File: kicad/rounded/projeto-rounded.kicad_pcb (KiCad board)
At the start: 2 copper layers, 123.2 x 127 mm, 57 parts, among them Q1 BTA16-600B, Q2 BTA16-600B, U1 ESP-12E, U3v3 LM1117-3.3

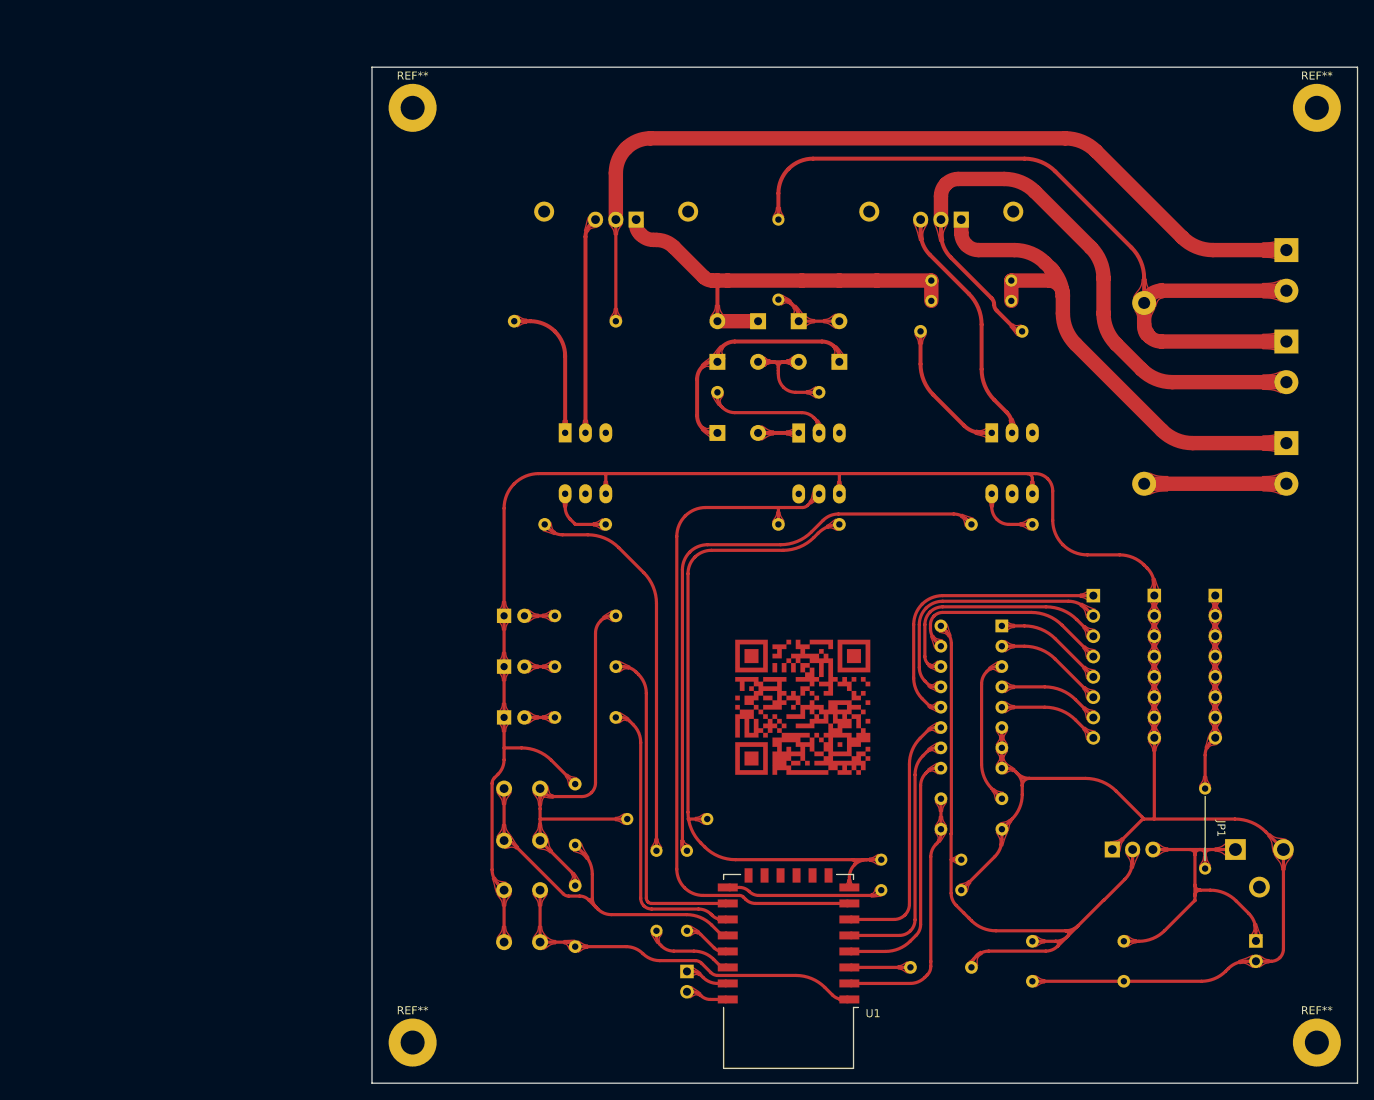
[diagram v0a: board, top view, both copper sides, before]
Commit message: Fix PCB
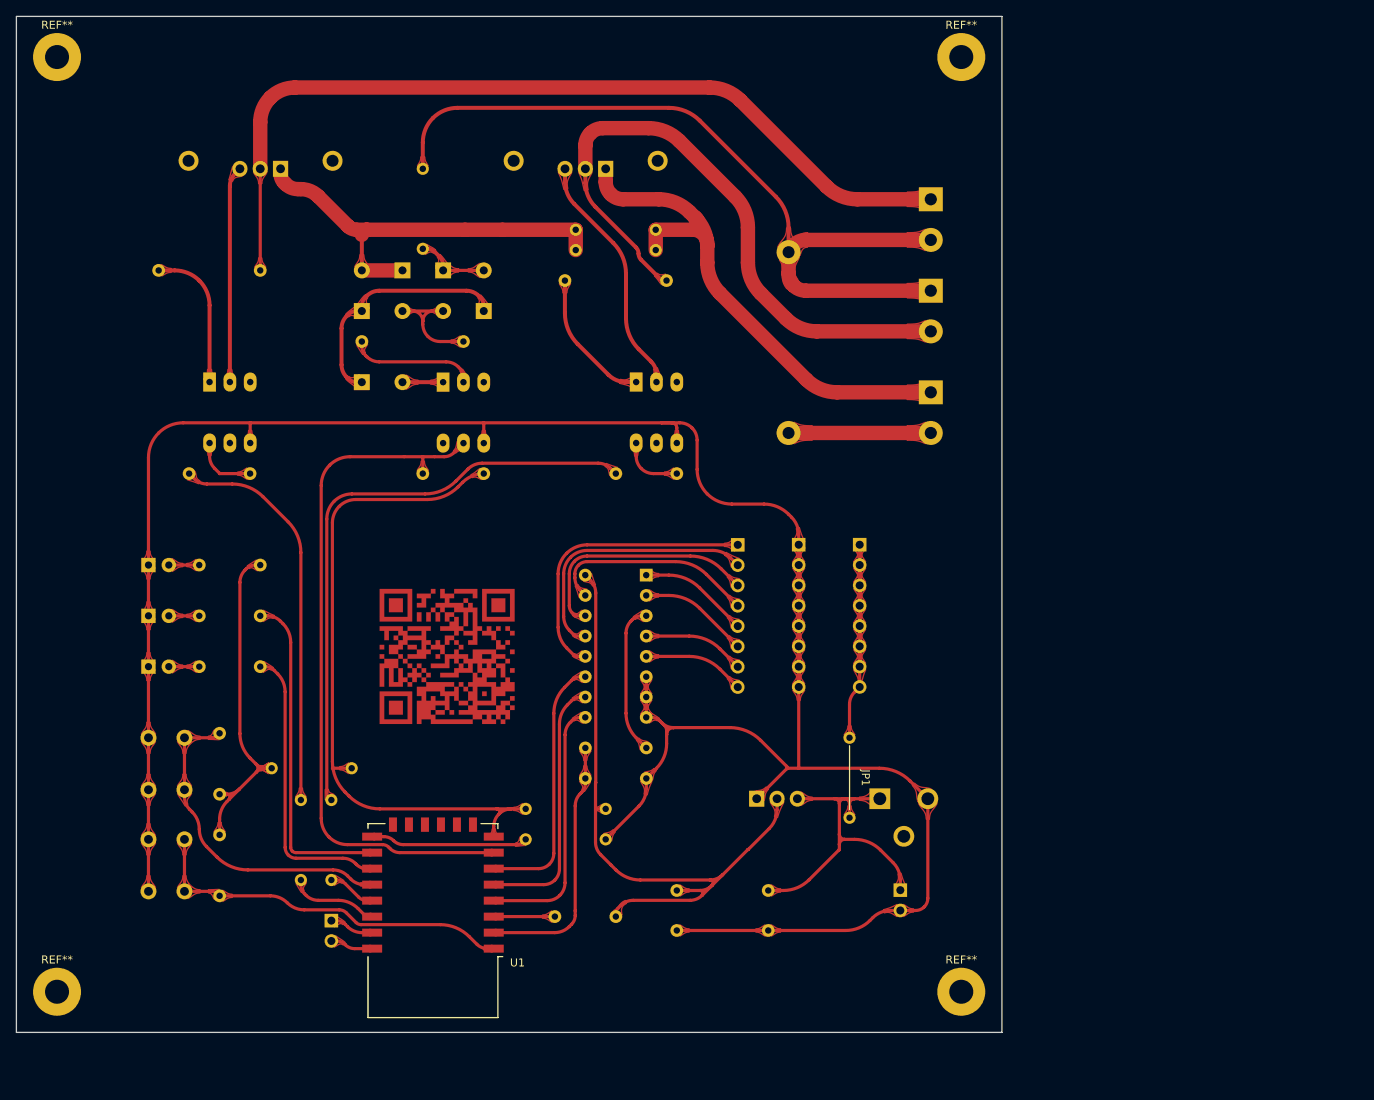
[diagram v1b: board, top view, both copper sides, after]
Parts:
- moved D2 44.9 mm to (137.2, 59.7)
- moved JP5 44.9 mm to (157.5, 127.0)
- moved JP6 44.9 mm to (147.5, 130.8)
- moved JP8 44.9 mm to (119.4, 125.9)
- moved Jpwr_sens1 44.9 mm to (189.2, 94.0)
- moved Q1 44.9 mm to (157.5, 47.0)
- moved Ren1 44.9 mm to (151.1, 140.5)
- moved Rtriac1 44.9 mm to (152.4, 61.0)
- moved Rtriac2 44.9 mm to (101.6, 59.7)
- moved U1 44.9 mm to (135.9, 141.0)
- moved Udet_0 44.9 mm to (137.2, 73.7)
- moved Uload1 44.9 mm to (161.3, 73.6)
- moved Don1 44.9 mm to (100.3, 96.5)
- moved Dss1 44.9 mm to (100.3, 102.9)
- moved Dwifi1 44.9 mm to (100.3, 109.2)
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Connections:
- Rexit1 pad 1: /exit_intr -> /3v3'2
- Rexit1 pad 2: GND -> /exit_intr
- SWexit1 pad 1: /3v3'2 -> /exit_intr
- SWexit1 pad 2: /exit_intr -> GND
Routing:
- net GND: track 309.9 -> 299.2 mm
- net /3v3'2: track 54.7 -> 44.7 mm
- net /exit_intr: track 47.9 -> 41.1 mm
- net Net-(D2-Pad2): track 17.0 -> 15.6 mm
- net /AC2': track 53.4 -> 54.4 mm
- net /multiplex_C: track 31.6 -> 32.4 mm
